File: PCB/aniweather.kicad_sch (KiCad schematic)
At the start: 24 parts, among them SW1 SW_DIP_x01, SW2 SW_Push, U5 TPS63001

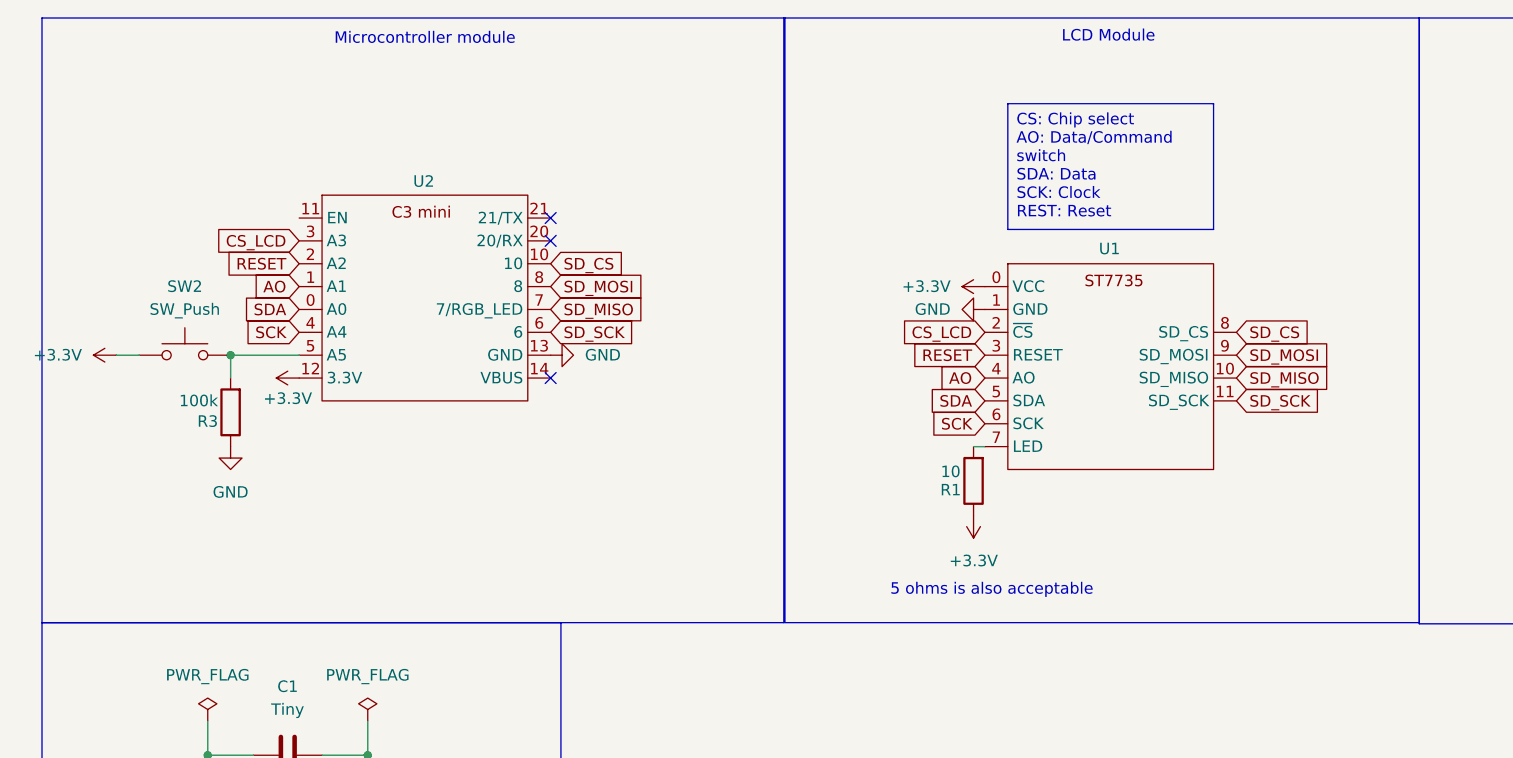
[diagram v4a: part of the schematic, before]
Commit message: Reroute board
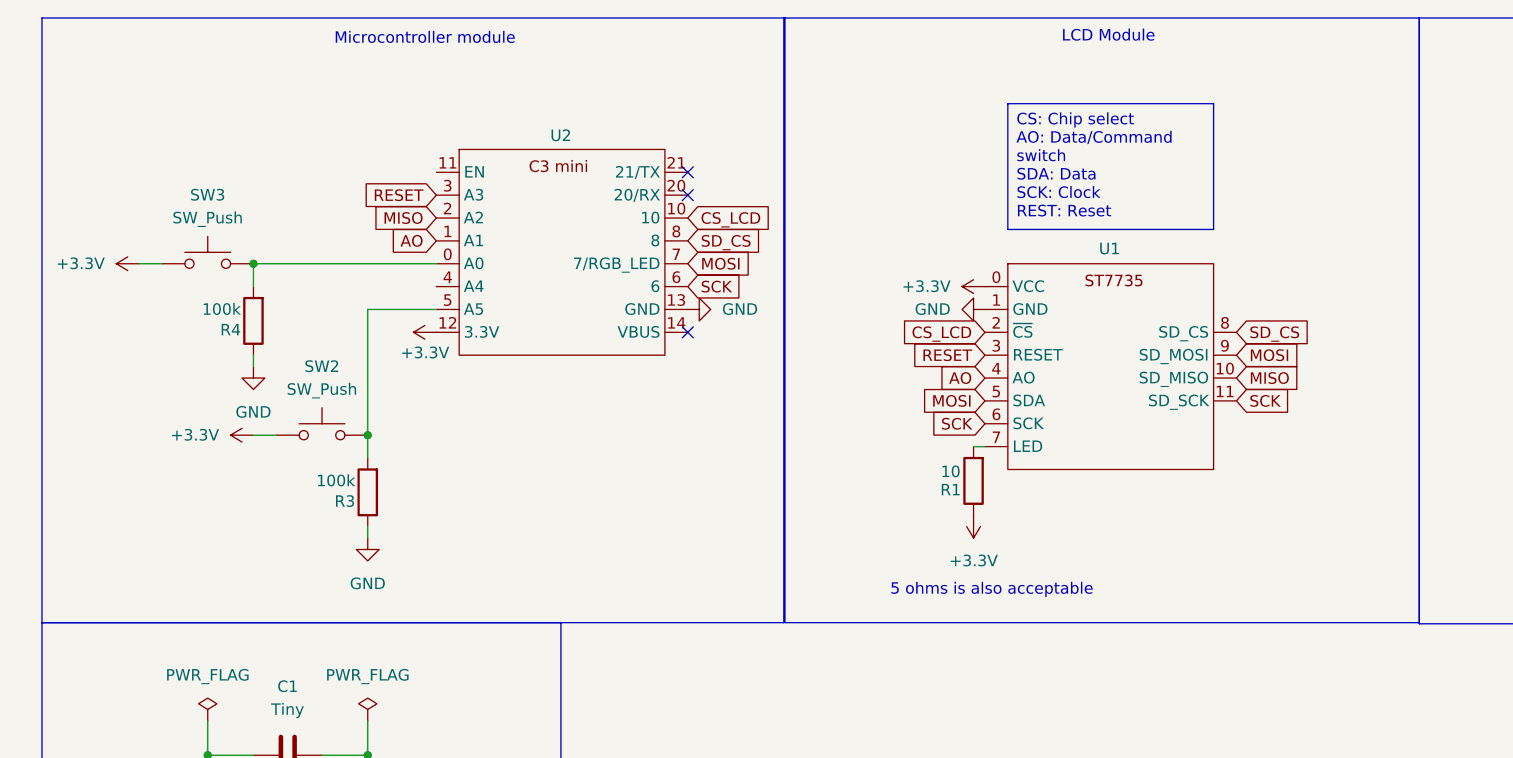
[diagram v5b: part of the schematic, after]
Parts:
- added R4: 100k, Resistor_THT:R_Axial_DIN0207_L6.3mm_D2.5mm_P10.16mm_Horizontal, symbol Device:R
- added SW3: SW_Push, Button_Switch_THT:SW_PUSH_6mm, symbol Switch:SW_Push
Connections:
- net SD_SCK is gone; now on net SCK: U1.11 (SD_SCK), U2.6
- net +3.3V: now also SW3.1
- net CS_LCD: now also U2.10; no longer U2.3 (A3)
- net GND: now also R4.1
- net RESET: now also U2.3 (A3); no longer U2.2 (A2)
- net SCK: no longer U2.4 (A4)
- net SD_CS: now also U2.8; no longer U2.10
- net SDA: no longer names the net of U2.0 (A0)
- net SDA: now also R4.2, SW3.2; no longer U1.5 (SDA)
- net SD_MISO renamed MISO
- net MISO: now also U2.2 (A2); no longer U2.7 (7/RGB_LED)
- net SD_MOSI renamed MOSI
- net MOSI: now also U1.5 (SDA), U2.7 (7/RGB_LED); no longer U2.8
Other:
- moved on the sheet: R3, SW2, U2
